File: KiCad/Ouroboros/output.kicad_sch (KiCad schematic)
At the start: 14 parts, among them J1 AudioJack2, SW1 SW_DPDT_x2, U1 Opamp_Quad

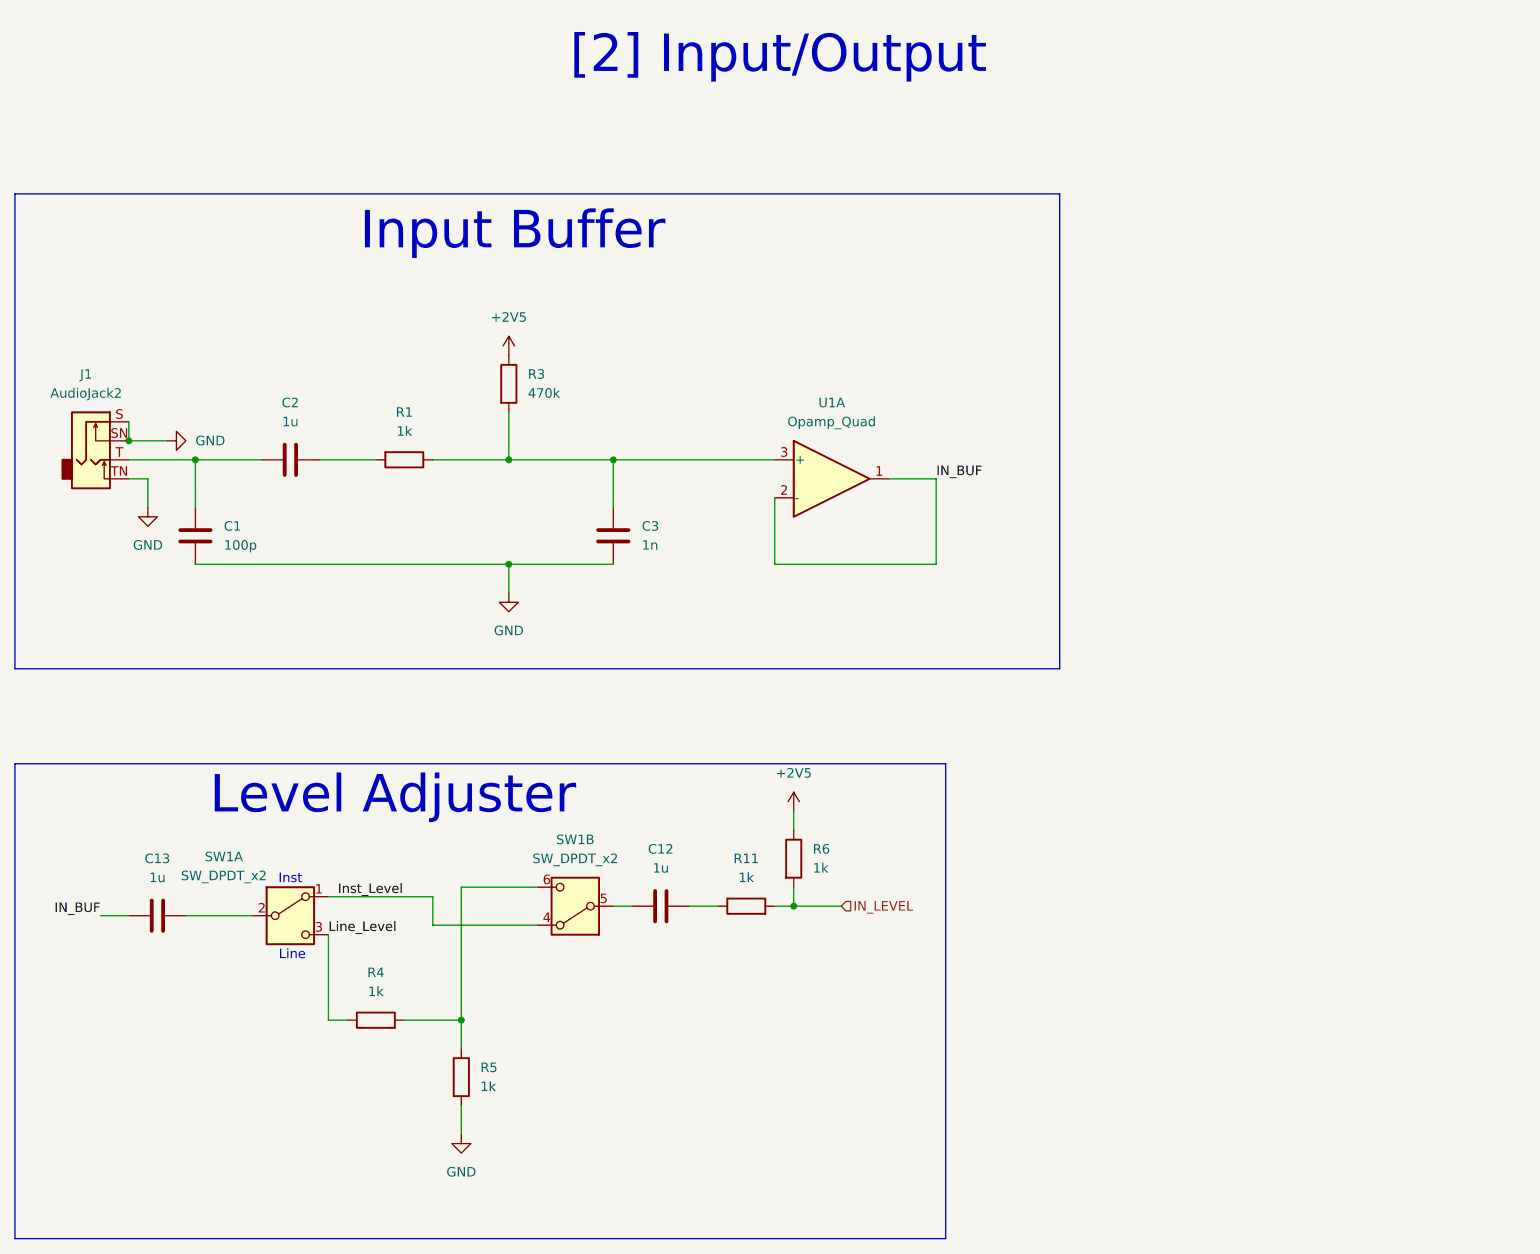
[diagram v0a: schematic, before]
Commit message: PCB Finished
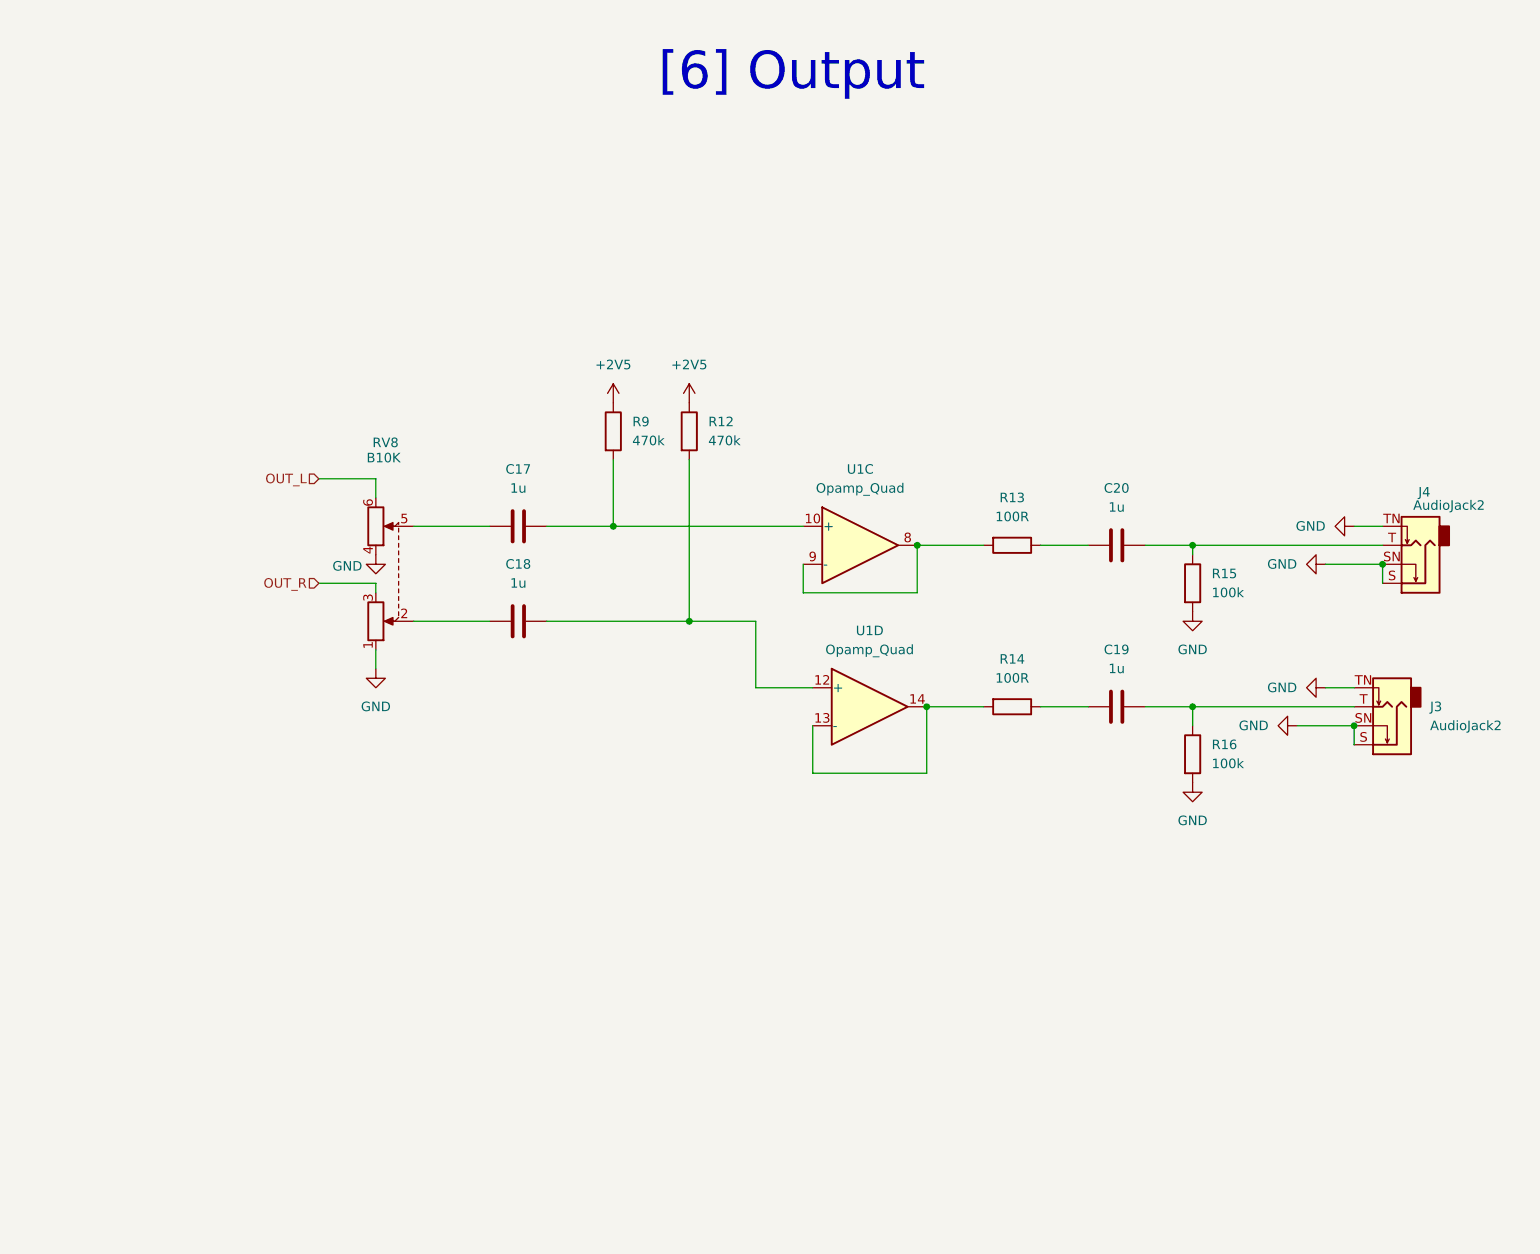
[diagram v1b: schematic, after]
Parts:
- removed C1: 100p, Capacitor_THT:C_Rect_L7.0mm_W3.5mm_P5.00mm, symbol Device:C
- removed C12, C13: 1u, Capacitor_THT:C_Rect_L7.0mm_W3.5mm_P5.00mm, symbol Device:C
- removed C2: 1u, Capacitor_THT:C_Rect_L7.0mm_W6.0mm_P5.00mm, symbol Device:C
- removed C3: 1n, Capacitor_THT:C_Rect_L7.0mm_W3.5mm_P5.00mm, symbol Device:C
- removed J1: AudioJack2, Connector_Audio:Jack_6.35mm_Neutrik_NMJ4HFD2_Horizontal, symbol Connector_Audio:NMJ4HFD2
- removed R1, R11, R4, R5, R6: 1k, Resistor_THT:R_Axial_DIN0207_L6.3mm_D2.5mm_P10.16mm_Horizontal, symbol Device:R
- removed R3: 470k, Resistor_THT:R_Axial_DIN0207_L6.3mm_D2.5mm_P10.16mm_Horizontal, symbol Device:R
- removed SW1: SW_DPDT_x2, Library:DPDT_Mini_Toggle, symbol Switch:SW_DPDT_x2
- removed U1: Opamp_Quad, Package_DIP:DIP-14_W7.62mm_Socket, symbol Amplifier_Operational:TL074
- added C17, C18, C19, C20: 1u, Capacitor_THT:C_Rect_L7.0mm_W6.0mm_P5.00mm, symbol Device:C
- added J3, J4: AudioJack2, Connector_Audio:Jack_6.35mm_Neutrik_NMJ4HFD2_Horizontal, symbol Connector_Audio:NMJ4HFD2
- added R12, R9: 470k, Resistor_THT:R_Axial_DIN0207_L6.3mm_D2.5mm_P10.16mm_Horizontal, symbol Device:R
- added R13, R14: 100R, Resistor_THT:R_Axial_DIN0207_L6.3mm_D2.5mm_P10.16mm_Horizontal, symbol Device:R
- added R15, R16: 100k, Resistor_THT:R_Axial_DIN0207_L6.3mm_D2.5mm_P10.16mm_Horizontal, symbol Device:R
- added RV8: B10K, Potentiometer_THT:Potentiometer_Alpha_RD902F-40-00D_Dual_Vertical, symbol Device:R_Potentiometer_Dual
- added U1: Opamp_Quad, Package_DIP:DIP-14_W7.62mm_Socket, symbol Amplifier_Operational:TL074
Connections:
- net +2V5: now also R12.1, R9.1
- net GND: now also J3.S, J3.SN, J3.TN, J4.S, J4.SN, J4.TN, R15.2, R16.2, RV8.1, RV8.4
- new net: C19.1, R14.1
- new net: R14.2, U1.13 (-), U1.14
- new net: C20.1, R13.1
- new net: C20.2, J4.T, R15.1
- new net: R13.2, U1.8, U1.9 (-)
- new net: C18.1, RV8.2
- new net: C17.1, RV8.5
- new net: C18.2, R12.2, U1.12 (+)
- new net: C17.2, R9.2, U1.10 (+)
- new net: C19.2, J3.T, R16.1
- new net OUT_L: RV8.6
- new net OUT_R: RV8.3
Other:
- note added: "[6] Output"
- note removed: "Input Buffer"
- note removed: "Inst"
- note removed: "Level Adjuster"
- note removed: "Line"
- note removed: "[2] Input/Output"
